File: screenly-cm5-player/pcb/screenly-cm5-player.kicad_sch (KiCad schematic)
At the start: 0 parts

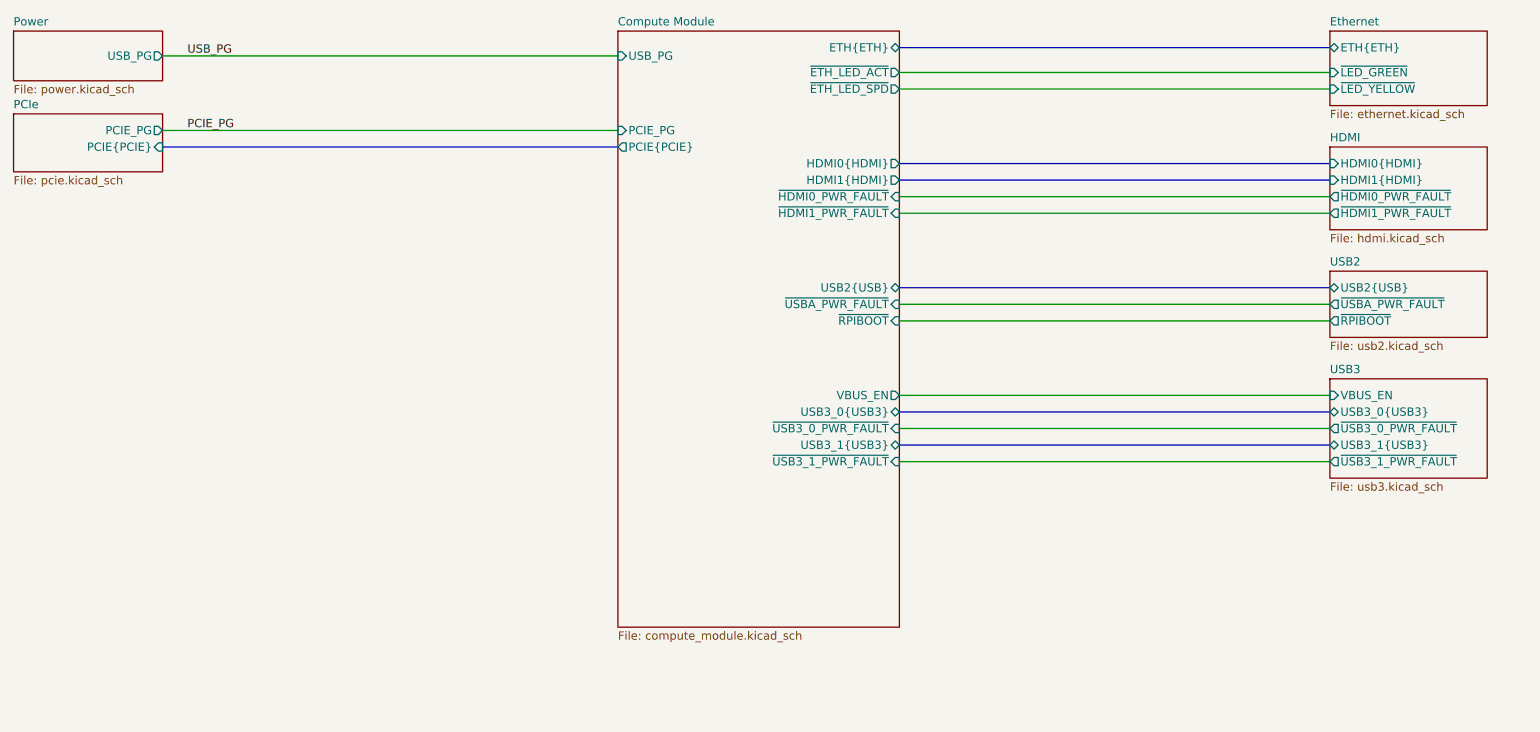
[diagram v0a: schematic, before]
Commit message: Finished schematics design.
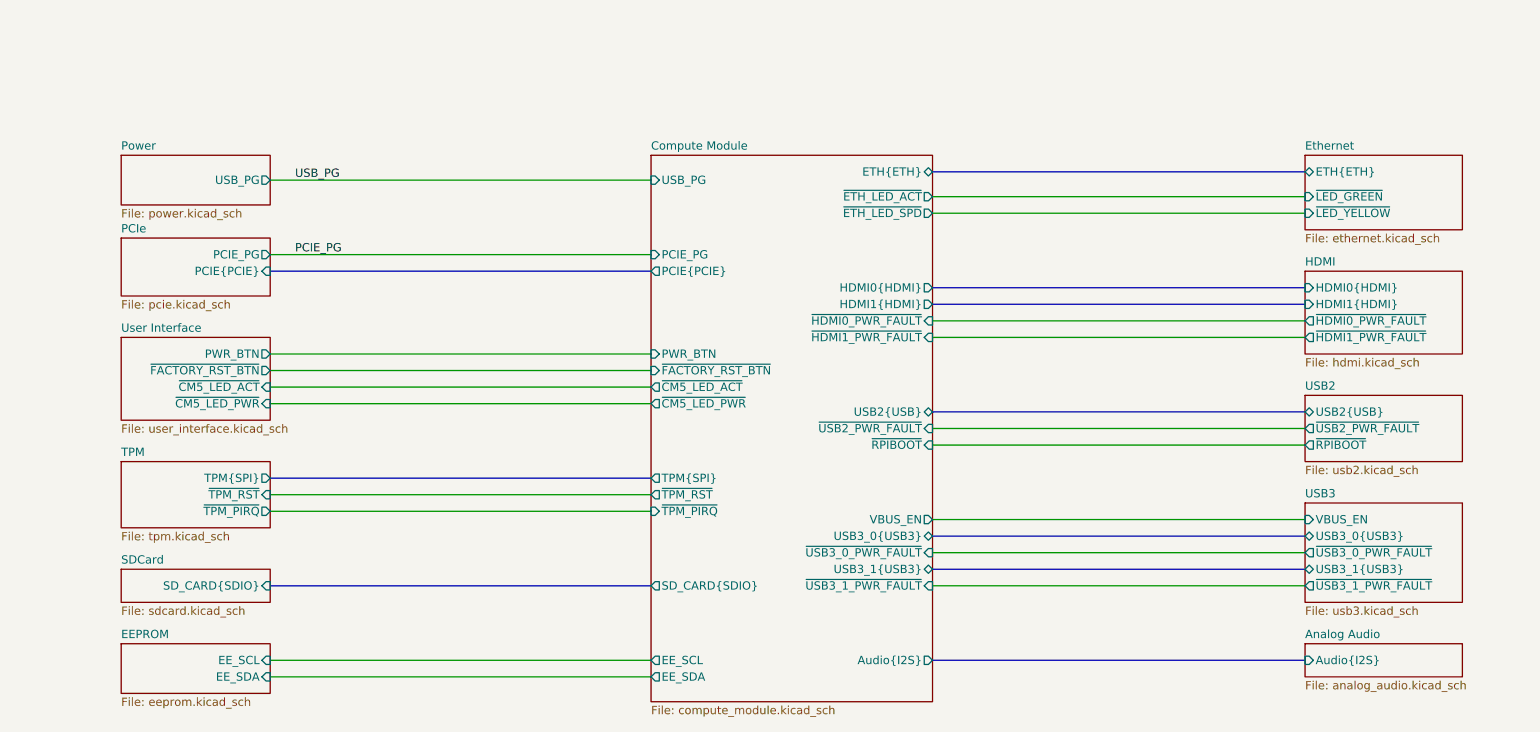
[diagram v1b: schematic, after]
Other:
- added sheet Analog Audio (analog_audio.kicad_sch)
- added sheet EEPROM (eeprom.kicad_sch)
- added sheet SDCard (sdcard.kicad_sch)
- added sheet TPM (tpm.kicad_sch)
- added sheet User Interface (user_interface.kicad_sch)
- sheet Compute Module ports: added Audio{I2S}, EE_SCL, EE_SDA, PWR_BTN, SD_CARD{SDIO}, TPM{SPI}, ~{CM5_LED_ACT}, ~{CM5_LED_PWR}, ~{FACTORY_RST_BTN}, ~{TPM_PIRQ}, ~{TPM_RST}, ~{USB2_PWR_FAULT}; removed ~{USBA_PWR_FAULT}
- sheet USB2 ports: added ~{USB2_PWR_FAULT}; removed ~{USBA_PWR_FAULT}
